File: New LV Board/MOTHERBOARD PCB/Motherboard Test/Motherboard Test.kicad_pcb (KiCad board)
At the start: 2 copper layers, 36 parts, among them J1 PH1-20-UA, J2 PH1-10-UA

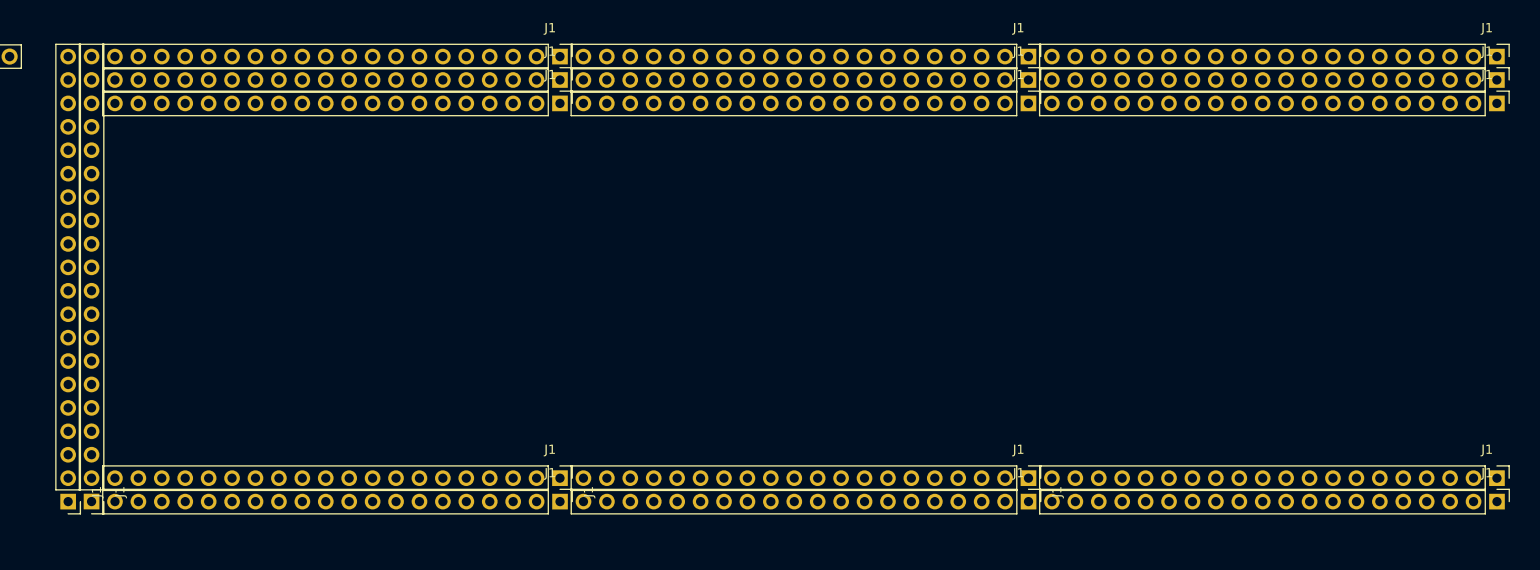
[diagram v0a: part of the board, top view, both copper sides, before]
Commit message: Not sure what changed, probably just opening a file
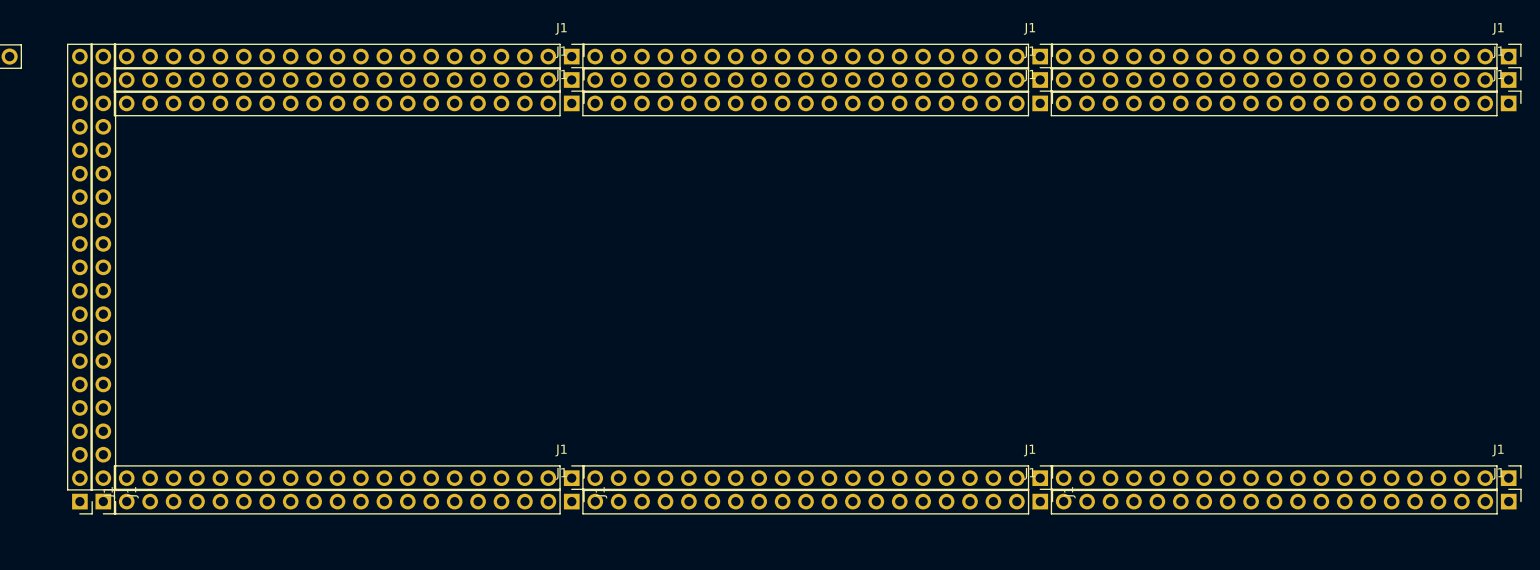
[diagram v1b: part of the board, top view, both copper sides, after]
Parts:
- moved J1 1.28 mm to (215.9, 16.5)
- moved J1 1.28 mm to (215.9, 62.2)
- moved J1 1.28 mm to (215.9, 19.1)
- moved J1 1.28 mm to (114.3, 16.5)
- moved J1 1.28 mm to (114.3, 14.0)
- moved J1 1.28 mm to (114.3, 59.7)
- moved J1 1.28 mm to (165.1, 19.1)
- moved J1 1.28 mm to (165.1, 16.5)
- moved J1 1.28 mm to (165.1, 14.0)
- moved J1 1.28 mm to (165.1, 59.7)
- moved J1 1.28 mm to (215.9, 59.7)
- moved J1 1.28 mm to (215.9, 14.0)
- moved J1 1.28 mm to (114.3, 19.1)
- moved J1 1.27 mm to (61.0, 62.2)
- moved J1 1.27 mm to (63.5, 62.2)
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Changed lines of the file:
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@@
 	(footprint "Connector_PinHeader_2.54mm:PinHeader_1x20_P2.54mm_Vertical"
 		(layer "F.Cu")
-		(at 163.83 62.23 -90)
+		(at 165.105 62.23 -90)
 		(descr "Through hole straight pin header, 1x20, 2.54mm pitch, single row")
 		(tags "Through hole pin header THT 1x20 2.54mm single row")
@@
 	(footprint "Connector_PinHeader_2.54mm:PinHeader_1x20_P2.54mm_Vertical"
 		(layer "F.Cu")
-		(at 214.625 59.69 -90)
+		(at 215.9 59.69 -90)
 		(descr "Through hole straight pin header, 1x20, 2.54mm pitch, single row")
 		(tags "Through hole pin header THT 1x20 2.54mm single row")
@@
 	(footprint "Connector_PinHeader_2.54mm:PinHeader_1x20_P2.54mm_Vertical"
 		(layer "F.Cu")
-		(at 214.62 13.97 -90)
+		(at 215.895 13.97 -90)
 		(descr "Through hole straight pin header, 1x20, 2.54mm pitch, single row")
 		(tags "Through hole pin header THT 1x20 2.54mm single row")
@@
 	(footprint "Connector_PinHeader_2.54mm:PinHeader_1x20_P2.54mm_Vertical"
 		(layer "F.Cu")
-		(at 113.02 19.05 -90)
+		(at 114.295 19.05 -90)
 		(descr "Through hole straight pin header, 1x20, 2.54mm pitch, single row")
 		(tags "Through hole pin header THT 1x20 2.54mm single row")
@@
 	(footprint "Connector_PinHeader_2.54mm:PinHeader_1x20_P2.54mm_Vertical"
 		(layer "F.Cu")
-		(at 59.685 62.23 180)
+		(at 60.96 62.23 180)
 		(descr "Through hole straight pin header, 1x20, 2.54mm pitch, single row")
 		(tags "Through hole pin header THT 1x20 2.54mm single row")
@@
 	(footprint "Connector_PinHeader_2.54mm:PinHeader_1x20_P2.54mm_Vertical"
 		(layer "F.Cu")
-		(at 214.62 16.51 -90)
+		(at 215.895 16.51 -90)
 		(descr "Through hole straight pin header, 1x20, 2.54mm pitch, single row")
 		(tags "Through hole pin header THT 1x20 2.54mm single row")
@@
 	(footprint "Connector_PinHeader_2.54mm:PinHeader_1x20_P2.54mm_Vertical"
 		(layer "F.Cu")
-		(at 214.63 62.23 -90)
+		(at 215.905 62.23 -90)
 		(descr "Through hole straight pin header, 1x20, 2.54mm pitch, single row")
 		(tags "Through hole pin header THT 1x20 2.54mm single row")
@@
 	(footprint "Connector_PinHeader_2.54mm:PinHeader_1x20_P2.54mm_Vertical"
 		(layer "F.Cu")
-		(at 214.62 19.05 -90)
+		(at 215.895 19.05 -90)
 		(descr "Through hole straight pin header, 1x20, 2.54mm pitch, single row")
 		(tags "Through hole pin header THT 1x20 2.54mm single row")
@@
 	(footprint "Connector_PinHeader_2.54mm:PinHeader_1x20_P2.54mm_Vertical"
 		(layer "F.Cu")
-		(at 62.225 62.225 180)
+		(at 63.5 62.225 180)
 		(descr "Through hole straight pin header, 1x20, 2.54mm pitch, single row")
 		(tags "Through hole pin header THT 1x20 2.54mm single row")
@@
 	(footprint "Connector_PinHeader_2.54mm:PinHeader_1x20_P2.54mm_Vertical"
 		(layer "F.Cu")
-		(at 113.02 16.51 -90)
+		(at 114.295 16.51 -90)
 		(descr "Through hole straight pin header, 1x20, 2.54mm pitch, single row")
 		(tags "Through hole pin header THT 1x20 2.54mm single row")
@@
 	(footprint "Connector_PinHeader_2.54mm:PinHeader_1x20_P2.54mm_Vertical"
 		(layer "F.Cu")
-		(at 113.02 13.97 -90)
+		(at 114.295 13.97 -90)
 		(descr "Through hole straight pin header, 1x20, 2.54mm pitch, single row")
 		(tags "Through hole pin header THT 1x20 2.54mm single row")
@@
 	(footprint "Connector_PinHeader_2.54mm:PinHeader_1x20_P2.54mm_Vertical"
 		(layer "F.Cu")
-		(at 113.02 59.69 -90)
+		(at 114.295 59.69 -90)
 		(descr "Through hole straight pin header, 1x20, 2.54mm pitch, single row")
 		(tags "Through hole pin header THT 1x20 2.54mm single row")
@@
 	(footprint "Connector_PinHeader_2.54mm:PinHeader_1x20_P2.54mm_Vertical"
 		(layer "F.Cu")
-		(at 163.82 19.05 -90)
+		(at 165.095 19.05 -90)
 		(descr "Through hole straight pin header, 1x20, 2.54mm pitch, single row")
 		(tags "Through hole pin header THT 1x20 2.54mm single row")
@@
 	(footprint "Connector_PinHeader_2.54mm:PinHeader_1x20_P2.54mm_Vertical"
 		(layer "F.Cu")
-		(at 163.82 16.51 -90)
+		(at 165.095 16.51 -90)
 		(descr "Through hole straight pin header, 1x20, 2.54mm pitch, single row")
 		(tags "Through hole pin header THT 1x20 2.54mm single row")
@@
 	(footprint "Connector_PinHeader_2.54mm:PinHeader_1x20_P2.54mm_Vertical"
 		(layer "F.Cu")
-		(at 113.025 62.23 -90)
+		(at 114.3 62.23 -90)
 		(descr "Through hole straight pin header, 1x20, 2.54mm pitch, single row")
 		(tags "Through hole pin header THT 1x20 2.54mm single row")
@@
 	(footprint "Connector_PinHeader_2.54mm:PinHeader_1x20_P2.54mm_Vertical"
 		(layer "F.Cu")
-		(at 163.82 13.97 -90)
+		(at 165.095 13.97 -90)
 		(descr "Through hole straight pin header, 1x20, 2.54mm pitch, single row")
 		(tags "Through hole pin header THT 1x20 2.54mm single row")
@@
 	(footprint "Connector_PinHeader_2.54mm:PinHeader_1x20_P2.54mm_Vertical"
 		(layer "F.Cu")
-		(at 163.825 59.69 -90)
+		(at 165.1 59.69 -90)
 		(descr "Through hole straight pin header, 1x20, 2.54mm pitch, single row")
 		(tags "Through hole pin header THT 1x20 2.54mm single row")
@@
 	)
 	(gr_text "J1"
-		(at 116.13 61.165 90)
+		(at 117.405 61.165 90)
 		(layer "F.SilkS")
 		(effects
@@
 	)
 	(gr_text "J1"
-		(at 166.93 61.165 90)
+		(at 168.205 61.165 90)
 		(layer "F.SilkS")
 		(effects
